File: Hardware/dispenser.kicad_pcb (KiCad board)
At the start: 2 copper layers, 76.4 x 46.2 mm, 59 parts, among them J1 Vin, J2 encoder+btn, J3 YuMi_interface, J4 Motor, J5 Limitswitches, U1 SN74LVC1G14, U2 LM2675, U3 PC817, U4 ATMEGA328P-AU-Arduino, U5 PC817, U6 A4973, U7 PC817, U8 SN74LVC1G14, U9 SN74LVC1G14, Y1 8MHZ

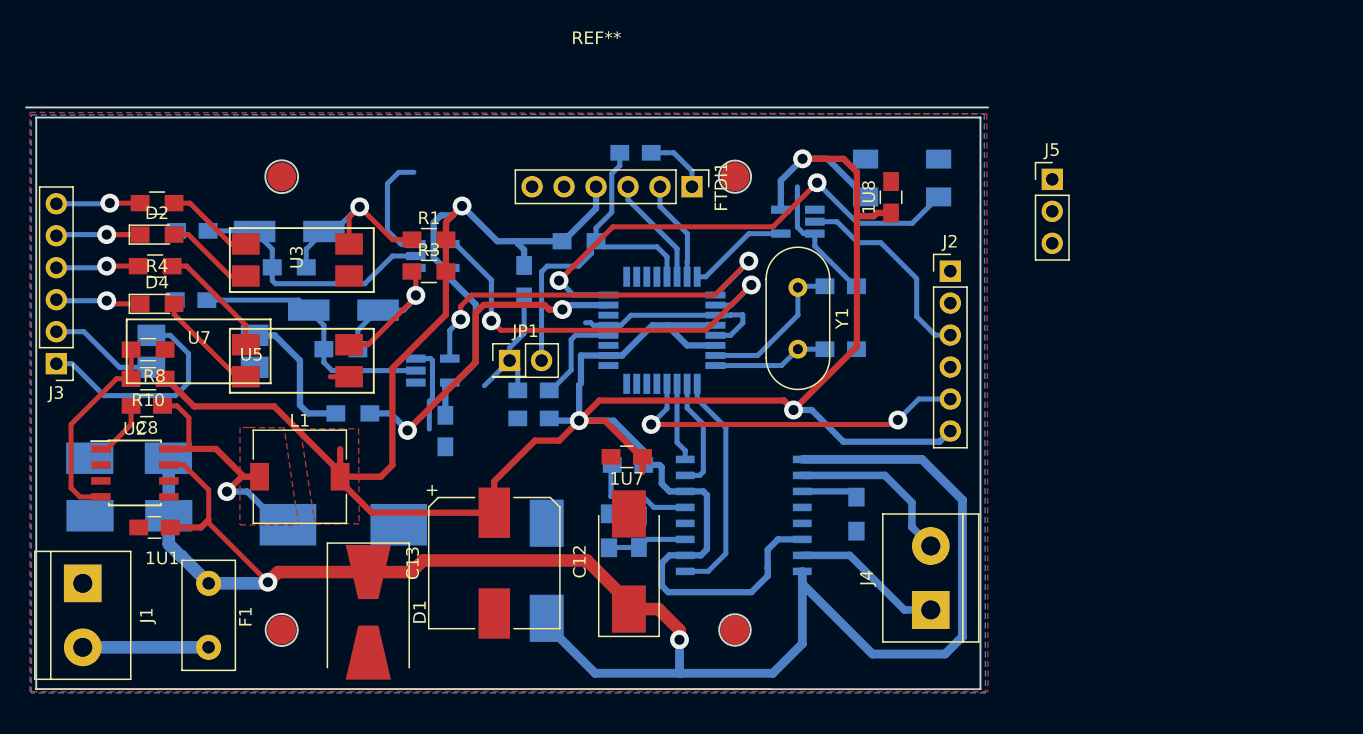
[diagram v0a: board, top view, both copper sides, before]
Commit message: sync old atmega files
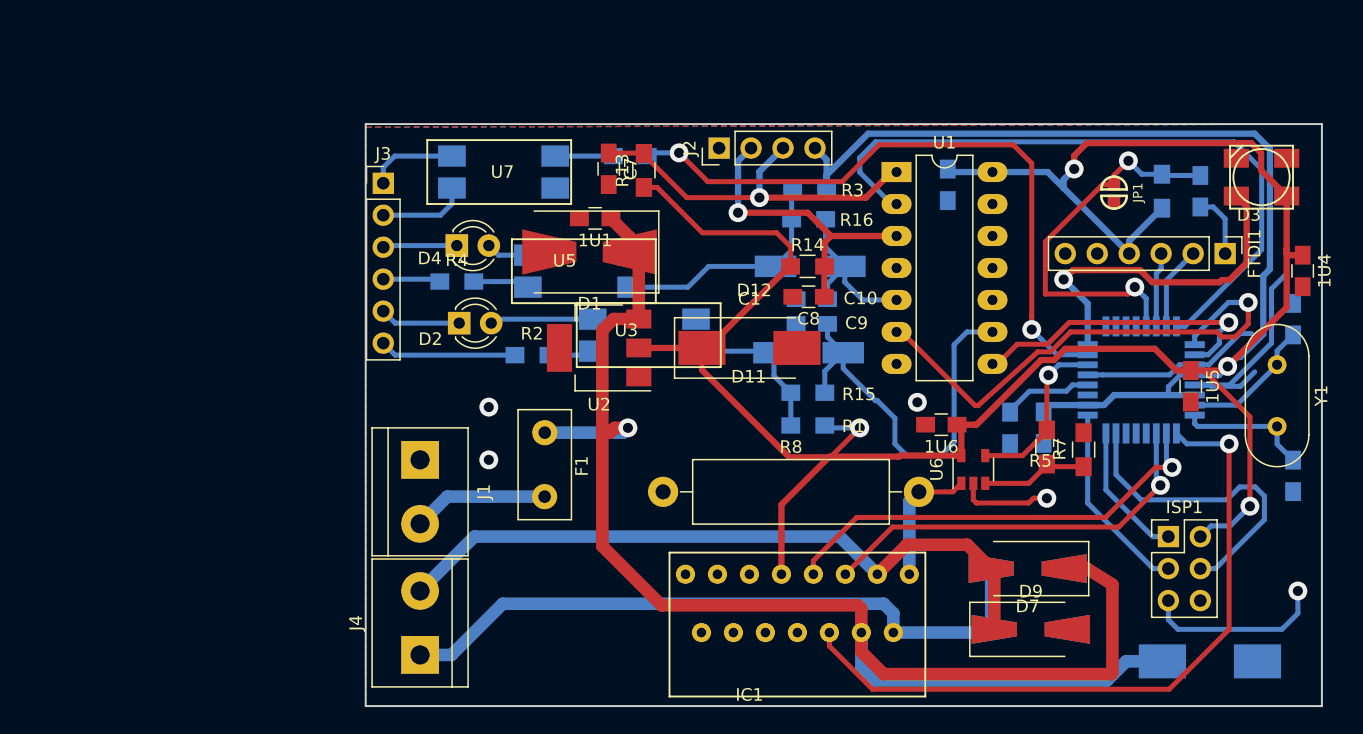
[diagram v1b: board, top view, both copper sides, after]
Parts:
- removed 1U3, 1U7: 0,1U, Capacitors_SMD:C_0805_HandSoldering
- removed C11: 470pFC, Capacitors_SMD:C_0805_HandSoldering
- removed C12: 47uf, Capacitors_Tantalum_SMD:CP_Tantalum_Case-D_EIA-7343-31_Hand
- removed C13: 330Uf, Capacitors_SMD:CP_Elec_10x10
- removed D5: D_Schottky, Diodes_SMD:D_SMC_Handsoldering
- removed J5: Limitswitches, Pin_Headers:Pin_Header_Straight_1x03_Pitch2.54mm
- removed L1: 47uH, Inductors_SMD:L_7.3x7.3_H4.5
- removed R10: 3K, Resistors_SMD:R_0805_HandSoldering
- removed REF**: Enclosure_ebay_82x52x35, Libs:Enclosure_ebay_82x52x35
- removed U8, U9: SN74LVC1G14, TO_SOT_Packages_SMD:SOT-23-5_HandSoldering
- added 1U6: 0,1U, Capacitors_SMD:C_0805_HandSoldering, F.Cu at (186.7, 120.4)
- added D6: D, Diodes_SMD:D_SMA-SMB_Universal_Handsoldering, B.Cu at (193.5, 131.8)
- added D7: D, Diodes_SMD:D_SMA-SMB_Universal_Handsoldering, F.Cu at (193.5, 131.8)
- added D8: D, Diodes_SMD:D_SMA-SMB_Universal_Handsoldering, B.Cu at (193.8, 136.7)
- added D9: D, Diodes_SMD:D_SMA-SMB_Universal_Handsoldering, F.Cu at (193.8, 136.7)
- added IC1: L298N, Libs:Multiwatt15_V, F.Cu at (172.7, 136.9)
- added ISP1: ISP-header, Pin_Headers:Pin_Header_Straight_2x03_Pitch2.54mm, F.Cu at (204.7, 129.3)
- added R13: 100K, Resistors_SMD:R_0805_HandSoldering, F.Cu at (163.1, 100.2)
- added R14: 100K, Resistors_SMD:R_0805_HandSoldering, F.Cu at (176.1, 107.8)
- 1U1: value 0.1uf -> 1U
- 1U4, 1U5, D3: moved to F.Cu
- 1U8, R1, R2, R3, R4, U3, U5: moved to B.Cu
- C1: value 4.7uF tant -> 22uf; footprint Capacitors_Tantalum_SMD:CP_Tantalum_Case-C_EIA-6032-28_Hand -> Capacitors_Tantalum_SMD:CP_Tantalum_Case-D_EIA-7343-31_Hand; moved to F.Cu
- C5: value 47uf -> 22uf
- C7: value 4.7uF tant -> 47nF; footprint Capacitors_Tantalum_SMD:CP_Tantalum_Case-C_EIA-6032-28_Hand -> Capacitors_SMD:C_0805_HandSoldering; moved to F.Cu
- C8: value 10nf -> 47nF
- D2, D4: footprint LEDs:LED_0805_HandSoldering -> LEDs:LED_D3.0mm
- J2: value encoder+btn -> encoder_in; footprint Pin_Headers:Pin_Header_Straight_1x06_Pitch2.54mm -> Socket_Strips:Socket_Strip_Straight_1x04_Pitch2.54mm
- JP1: footprint Pin_Headers:Pin_Header_Straight_2x01_Pitch2.54mm -> jumper:SOLDER-JUMPER_1-WAY
- R5: value 30K -> 330K; moved to F.Cu
- R7: value 12R -> 6k8; moved to F.Cu
- R8: value 1K -> 1R; footprint Resistors_SMD:R_0805_HandSoldering -> Resistors_THT:R_Axial_DIN0516_L15.5mm_D5.0mm_P20.32mm_Horizontal
- U1: value SN74LVC1G14 -> 74HC14; footprint TO_SOT_Packages_SMD:SOT-23-5_HandSoldering -> Housings_DIP:DIP-14_W7.62mm_LongPads; moved to F.Cu
- U2: value LM2675 -> AMS117-5.0; footprint Housings_SOIC:SOIC-8_3.9x4.9mm_Pitch1.27mm -> TO_SOT_Packages_SMD:SOT-223
- U6: value A4973 -> LM321; footprint Housings_SOIC:SOIC-16W_7.5x10.3mm_Pitch1.27mm -> TO_SOT_Packages_SMD:SOT-23-5; moved to F.Cu
- moved 1U4 62.2 mm to (215.4, 108.2), turned to 270 degrees
- moved C8 53.3 mm to (176.1, 110.2)
- moved C5 53.2 mm to (208.0, 139.2), turned to 0 degrees
- moved C1 50.0 mm to (171.4, 114.3), turned to 0 degrees
- moved JP1 49.8 mm to (200.4, 102.0), turned to 90 degrees
- moved C9 49.8 mm to (176.4, 112.4)
- moved C10 49.3 mm to (176.4, 110.4)
- moved C7 47.0 mm to (160.3, 100.1), turned to 270 degrees
- moved R9 46.5 mm to (204.2, 101.9), turned to 90 degrees
- moved 1U5 45.1 mm to (206.5, 117.3), turned to 270 degrees
- moved C6 45.0 mm to (207.3, 101.9), turned to 90 degrees
- moved 1U2 42.9 mm to (194.8, 120.6)
- moved 1U1 42.7 mm to (159.2, 104.0)
- moved FTDI1 42.7 mm to (209.2, 106.8)
- moved R8 42.4 mm to (164.6, 125.7), turned to 0 degrees
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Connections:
- C1 pad 1: +24V -> VCC
- C7 pad 1: +24V -> Net-(C7-Pad1)
- C8 pad 2: Net-(C8-Pad2) -> GND
- D3 pad 1: GND -> Net-(D3-Pad1)
- D3 pad 2: LED -> Net-(D3-Pad2)
- D3 pad 3: VCC -> Net-(D3-Pad3)
- D3 pad 4: (no net) -> Net-(D3-Pad4)
- J2 pad 2: (no net) -> Net-(C8-Pad1)
- J2 pad 3: Net-(J2-Pad3) -> Net-(C7-Pad1)
- J2 pad 4: GND -> VCC
- J4 pad 1: Net-(J4-Pad1) -> Net-(D6-Pad2)
- J4 pad 2: Net-(J4-Pad2) -> Net-(D7-Pad2)
- R5 pad 1: Net-(C11-Pad1) -> Net-(R5-Pad1)
- R5 pad 2: GND -> Net-(R5-Pad2)
- R7 pad 1: Net-(R7-Pad1) -> Net-(R5-Pad2)
- R8 pad 2: Net-(R10-Pad2) -> current
- U1 pad 1: (no net) -> Net-(C7-Pad1)
- U1 pad 2: Net-(C9-Pad1) -> encA
- U1 pad 3: GND -> Net-(C8-Pad1)
- U1 pad 4: CMD -> Net-(U1-Pad4)
- U1 pad 5: VCC -> Net-(C10-Pad1)
- U2 pad 1: Net-(C8-Pad2) -> GND
- U2 pad 2: (no net) -> VCC
- U2 pad 3: (no net) -> +24V
- U2 pad 4: Net-(R10-Pad2) -> Net-(U2-Pad4)
- U4 pad 10: Phase -> in2
- U4 pad 11: Enable -> in1
- U4 pad 12: btn -> Net-(U4-Pad12)
- U4 pad 13: (no net) -> Net-(U4-Pad13)
- U4 pad 14: (no net) -> Net-(U4-Pad14)
- U4 pad 15: (no net) -> MOSI
- U4 pad 16: (no net) -> MISO
- U4 pad 17: (no net) -> SCK
- U4 pad 19: (no net) -> Net-(U4-Pad19)
- U4 pad 22: (no net) -> Net-(R5-Pad1)
- U4 pad 25: (no net) -> Net-(U4-Pad25)
- U4 pad 26: (no net) -> Net-(U4-Pad26)
- U4 pad 27: (no net) -> sda
- U4 pad 28: (no net) -> scl
- U4 pad 9: Break -> en
- U6 pad 1: Break -> current
- U6 pad 2: VCC -> GND
- U6 pad 3: Net-(C11-Pad1) -> Net-(R5-Pad2)
- U6 pad 4: GND -> Net-(R5-Pad1)
- U6 pad 5: GND -> VCC
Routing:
- net en: track 0.00 -> 55.5 mm, vias 0 -> 1
- net Net-(D7-Pad2): track 0.00 -> 55.1 mm
- net Net-(D6-Pad2): track 0.00 -> 54.5 mm
- net encA: track 8.59 -> 54.5 mm
- net in2: track 0.00 -> 35.9 mm, vias 0 -> 1
- net in1: track 0.00 -> 32.2 mm, vias 0 -> 1
- net Net-(C7-Pad1): track 0.00 -> 29.9 mm, vias 0 -> 1
- net btn: track 28.3 -> 0.00 mm, vias 2 -> 0
- net OUT: track 26.2 -> 51.9 mm
- net MOSI: track 0.00 -> 25.2 mm
- net GND: track 64.1 -> 40.6 mm, vias 0 -> 4
- net Break: track 18.2 -> 0.00 mm
- net reset_in: track 27.5 -> 45.3 mm, vias 0 -> 3
- net +24V: track 142.3 -> 124.5 mm, vias 2 -> 1
- net Net-(R10-Pad2): track 16.3 -> 0.00 mm
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- removed copper zone on F.Cu, net Net-(C8-Pad1)
- removed copper zone on F.Cu, net VCC
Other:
- board size 76.4 x 46.2 mm -> 75.9 x 46.2 mm
